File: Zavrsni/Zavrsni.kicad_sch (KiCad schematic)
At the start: 19 parts, among them J1 12V Source, J2 Input, J3 Output A, U1 LM78M05_TO220, U2 L298N

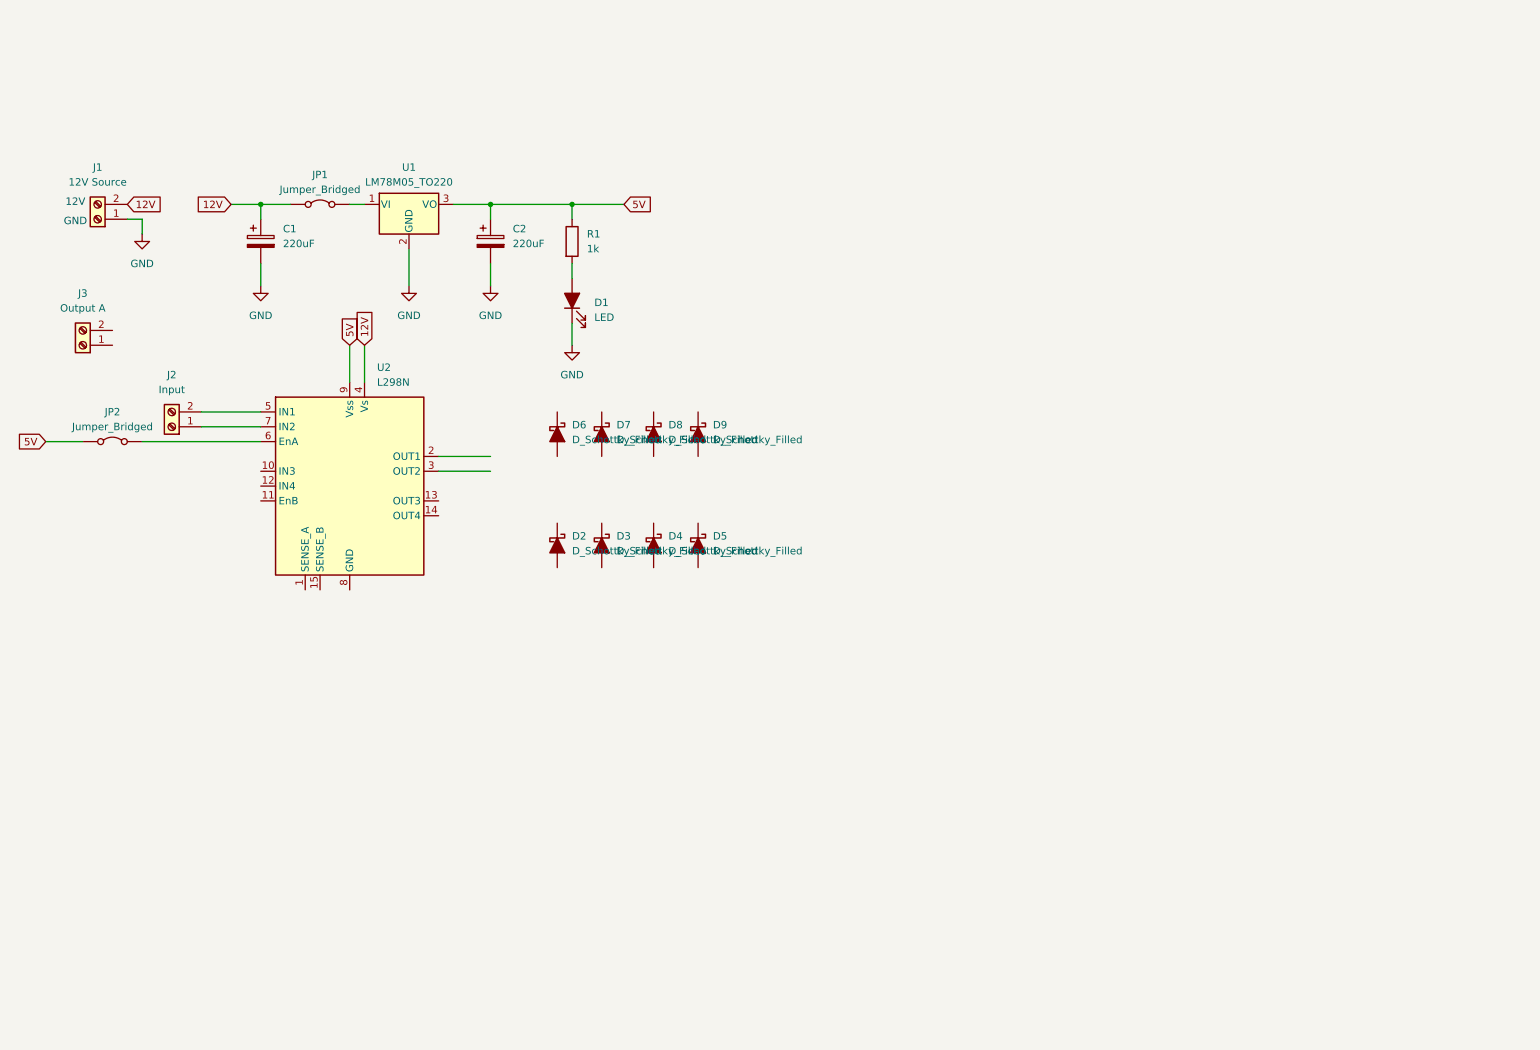
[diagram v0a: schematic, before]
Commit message: upd
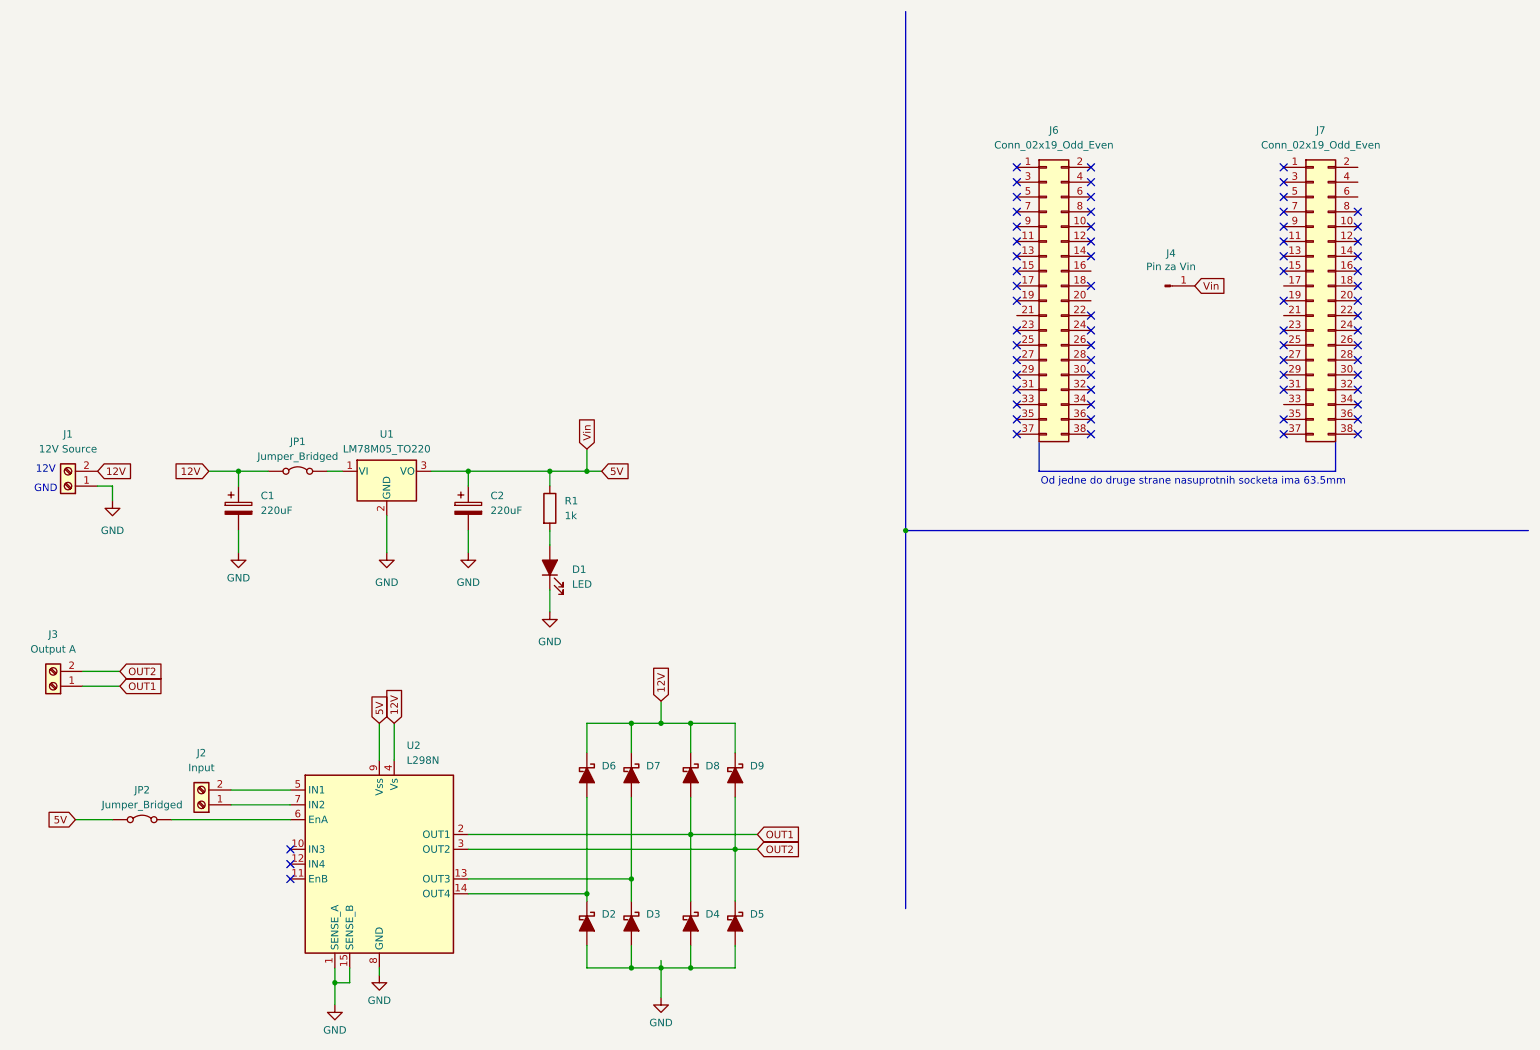
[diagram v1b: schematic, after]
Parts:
- added J4: Pin za Vin, Connector_PinHeader_2.54mm:PinHeader_1x01_P2.54mm_Vertical, symbol Connector:Conn_01x01_Pin
- added J6, J7: Conn_02x19_Odd_Even, Connector_PinSocket_2.54mm:PinSocket_2x19_P2.54mm_Vertical, symbol Connector_Generic:Conn_02x19_Odd_Even
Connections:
- net 12V: now also D6.1 (K), D7.1 (K), D8.1 (K), D9.1 (K)
- net 5V: now also J4.1 (Pin_1)
- net GND: now also D2.2 (A), D3.2 (A), D4.2 (A), D5.2 (A), U2.1 (SENSE_A), U2.15 (SENSE_B), U2.8 (GND)
- net OUT1: now reaches D4.1 (K)
- net OUT1: now also D8.2 (A), J3.1 (Pin_1), U2.2 (OUT1)
- net at U2.13 (OUT3): now also D3.1 (K), D7.2 (A)
- net at U2.14 (OUT4): now also D2.1 (K), D6.2 (A)
- net OUT2: now reaches U2.3 (OUT2)
- net OUT2: now also D5.1 (K), D9.2 (A), J3.2 (Pin_2)
- no-connect marks 0 -> 70
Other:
- note added: "Od jedne do druge strane nasuprotnih socketa ima 63.5mm"
- moved on the sheet: C1, C2, D1, D2, D3, D4, D5, D6, D7, D8, D9, J1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
